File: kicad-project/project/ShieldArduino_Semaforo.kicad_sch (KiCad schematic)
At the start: 78 parts, among them IC2 TPS563200DDCR, J1 Conn_01x01, J10 Conn_01x01, J11 Conn_01x01, J12 Conn_01x01, J13 Conn_01x01, J14 Conn_01x01, J15 Conn_01x01, J2 Conn_01x01, J3 Conn_01x01, J4 Conn_01x01, J5 Conn_01x01, J6 Conn_01x01, J7 Conn_01x01, J8 Conn_01x01, J9 Conn_01x01, K1 RELAY, P1 Power, P2 Analog, P3 Digital, P4 Digital, P5 CONN_01X01, P6 CONN_01X01, P7 CONN_01X01, P8 CONN_01X01, Q1 PMOS, Q2 NMOS, Q3 NMOS, Q4 NMOS, Q5 NMOS, U1 MCP2542FD-E/MF, U2 LM321

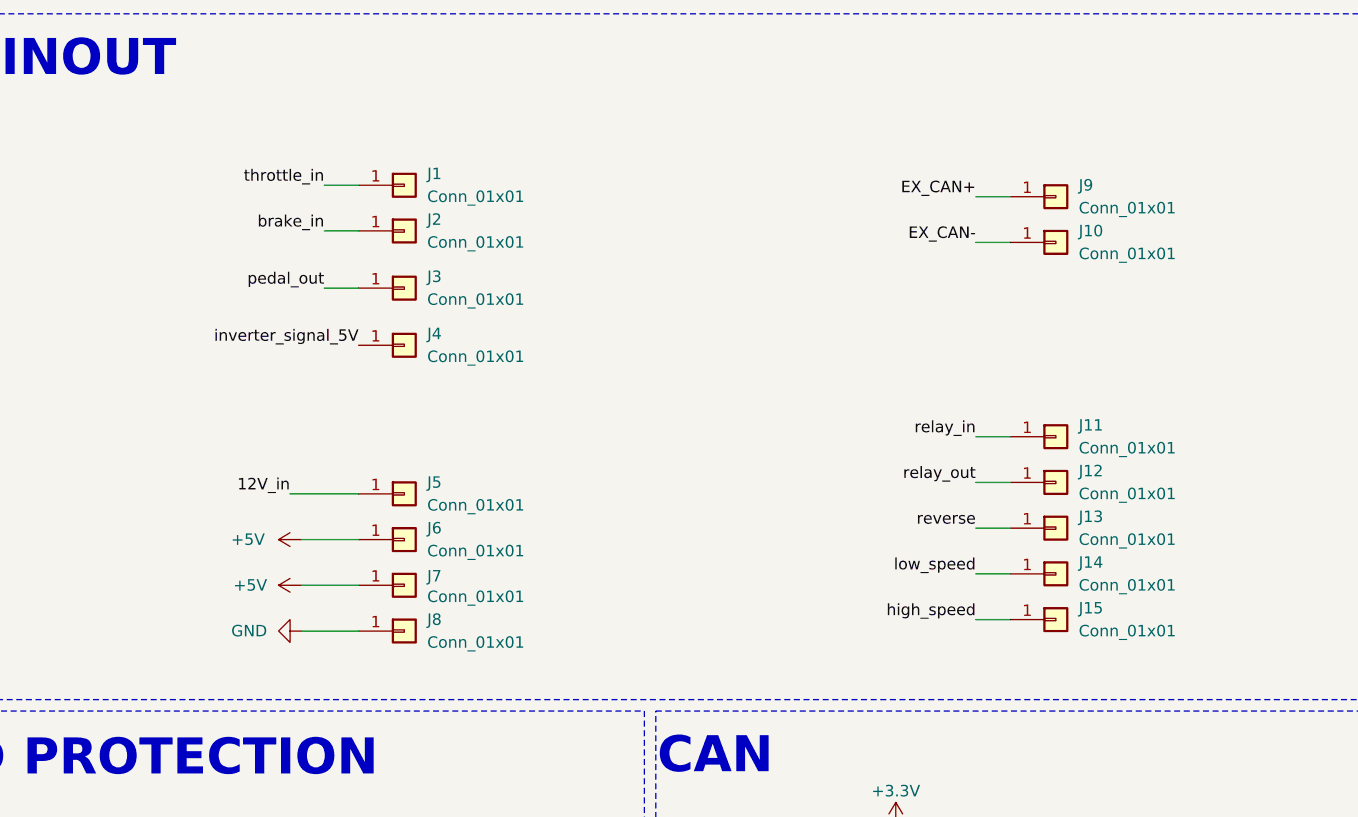
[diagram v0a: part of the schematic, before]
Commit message: kicad-pcb
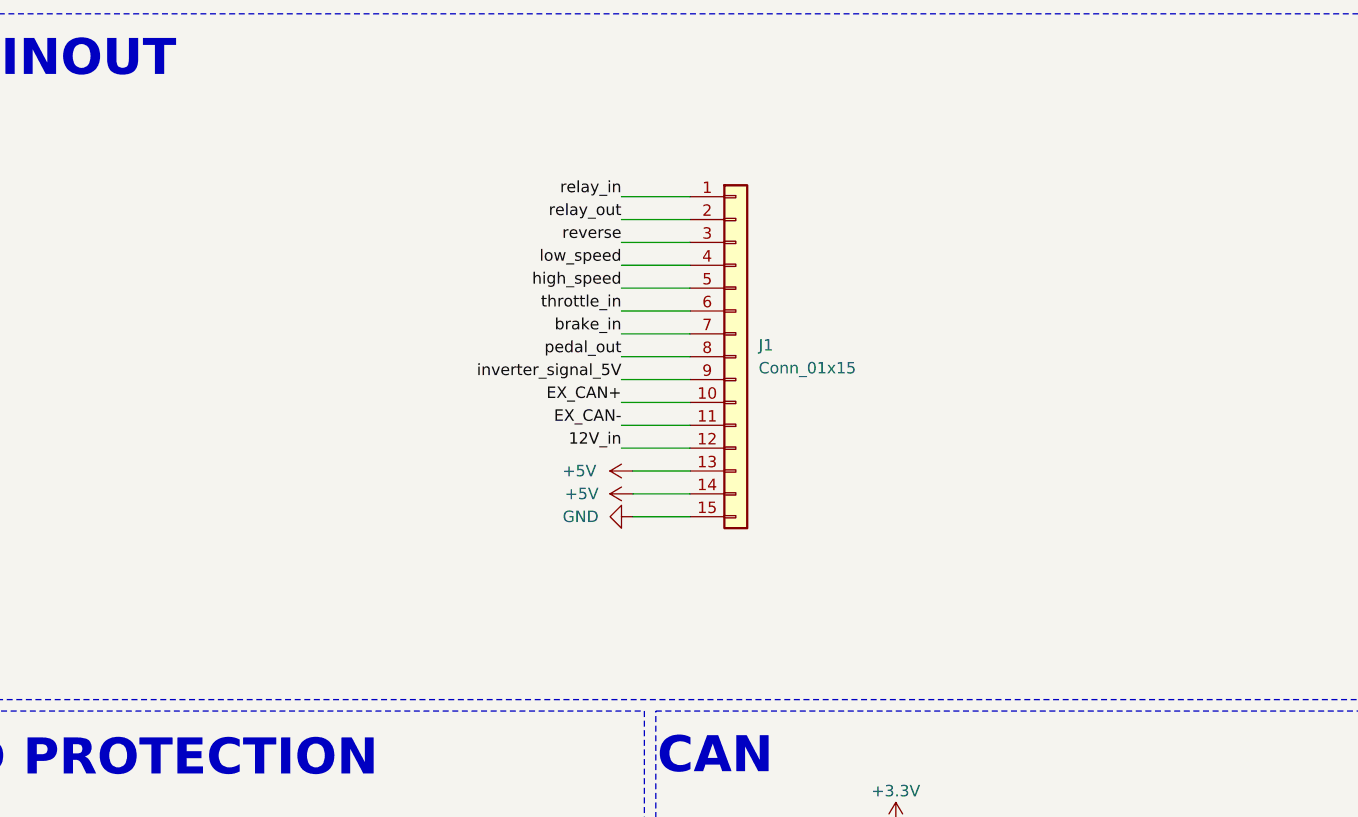
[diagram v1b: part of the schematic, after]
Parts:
- removed J1, J10, J11, J12, J13, J14, J15, J2, J3, J4, J5, J6, J7, J8, J9: Conn_01x01, Connector_Wire:SolderWire-0.1sqmm_1x01_D0.4mm_OD1mm_Relief, symbol Connector_Generic:Conn_01x01
- added J1: Conn_01x15, footprint:L17HTHES4R1C, symbol Connector_Generic:Conn_01x15
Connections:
- net  relay_in: now also J1.1 (Pin_1)
- net +5V: now also J1.13 (Pin_13), J1.14 (Pin_14)
- net 12V_in: now also J1.12 (Pin_12)
- net EX_CAN+: now also J1.10 (Pin_10)
- net EX_CAN-: now also J1.11 (Pin_11)
- net GND: now also J1.15 (Pin_15)
- net brake_in: now also J1.7 (Pin_7)
- net high_speed: now also J1.5 (Pin_5)
- net inverter_signal_5V: now also J1.9 (Pin_9)
- net low_speed: now also J1.4 (Pin_4)
- net pedal_out: now also J1.8 (Pin_8)
- net relay_out: now also J1.2 (Pin_2)
- net reverse: now also J1.3 (Pin_3)
- net throttle_in: now also J1.6 (Pin_6)
